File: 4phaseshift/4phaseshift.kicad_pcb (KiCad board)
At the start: 4 copper layers, 61 x 70 mm, 141 parts, among them J1 Conn_Coaxial, J10 Conn_Coaxial, J2 Conn_01x05_Pin, J3 Conn_Coaxial, J4 Conn_Coaxial, J7 Conn_Coaxial, J8 Conn_Coaxial, J9 Conn_Coaxial, U1 AMS1117, U10 TLV2372, U11 ADL5375-15ACPZ-WP, U12 TLV2372, U13 ADL5375-15ACPZ-WP, U14 SBB5089Z, U15 TLV2372, U16 ADL5375-15ACPZ-WP, U17 SBB5089Z, U18 TLV2372, U19 ADL5375-15ACPZ-WP, U2 AMS1117, U20 SBB5089Z, U3 YSGM556006, U7 DAC43608, U8 SBB5089Z, U9 SBB5089Z

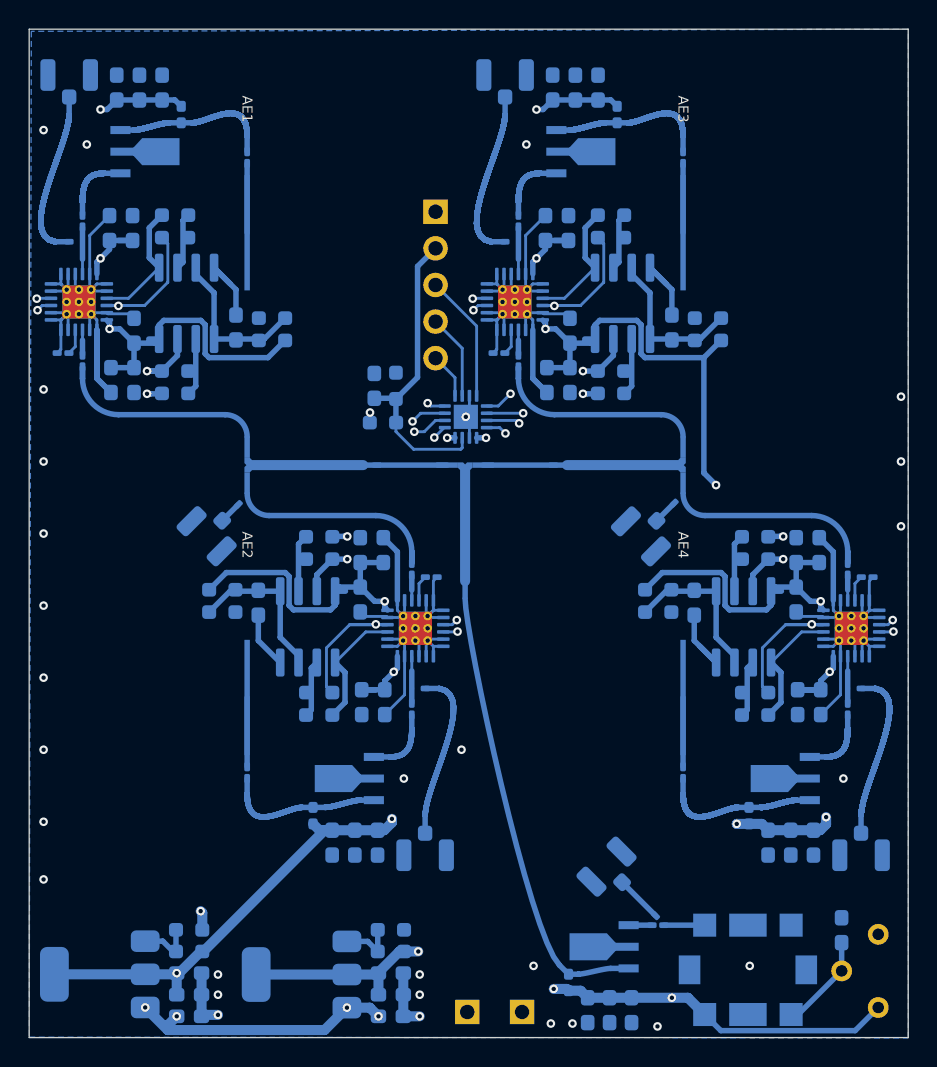
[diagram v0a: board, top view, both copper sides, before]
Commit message: saatvik mad
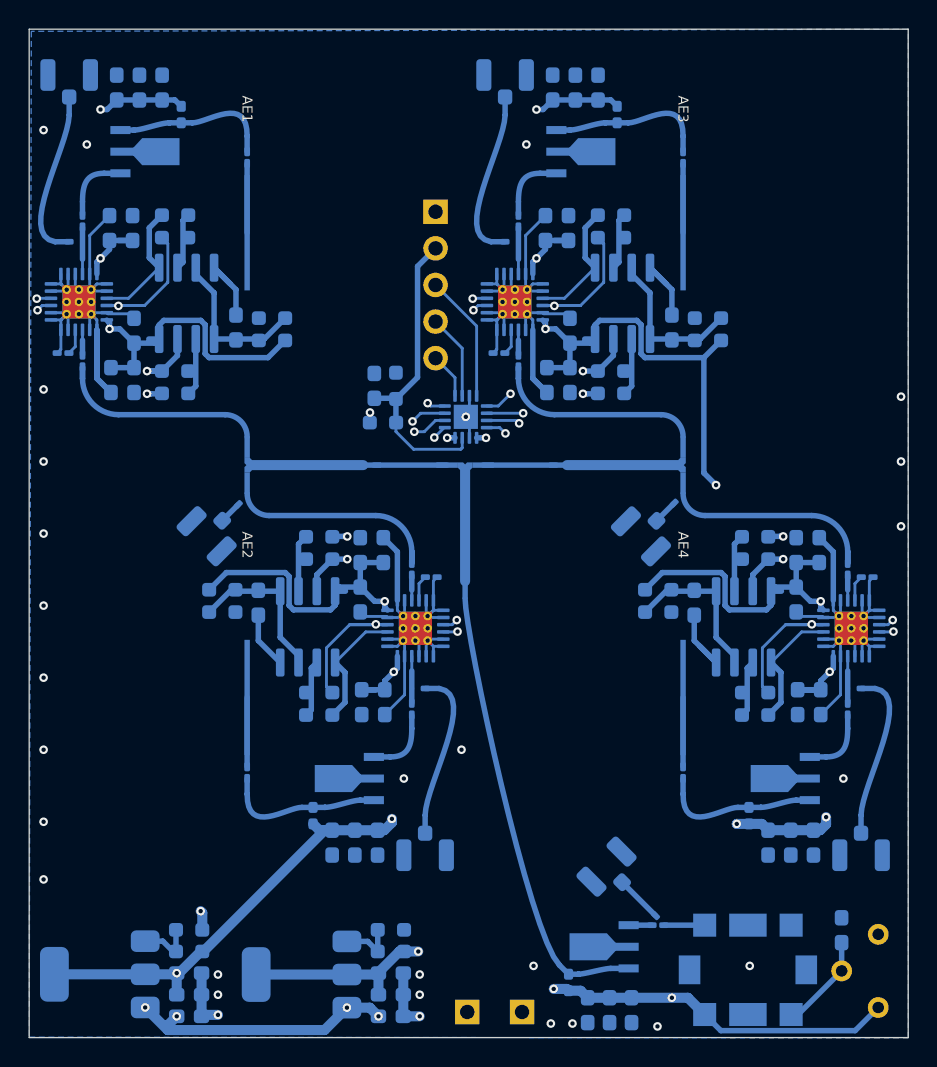
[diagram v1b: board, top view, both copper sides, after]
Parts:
- L1, L2, L3, L4, L5: value 82n -> 20n
- R1, R23: value 300 -> 560
- R10, R11, R12, R13, R14, R15, R16, R17, R18, R19, R20, R5, R6, R7, R8, R9: value 100k -> 10k
- R2, R24: value 100 -> 187
